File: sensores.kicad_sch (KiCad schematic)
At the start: 8 parts, among them U10 TCRT5000, U11 TCRT5000, U12 MPU-6050_module, U5 HC-Sr04, U6 HC-Sr04, U7 HC-Sr04, U8 KY-040, U9 KY-040

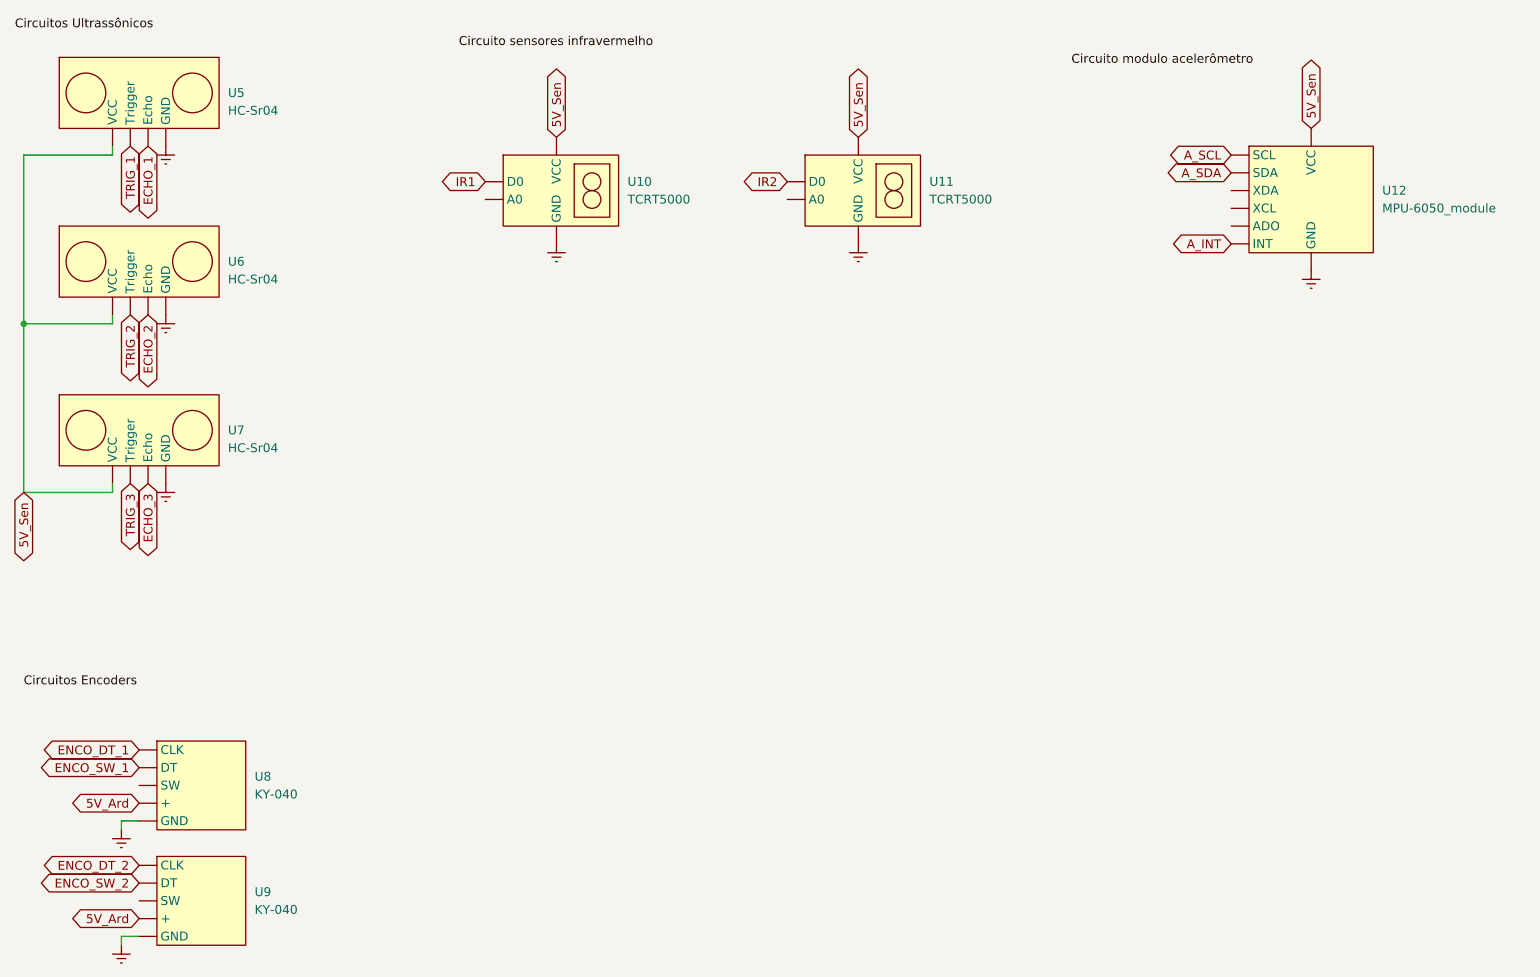
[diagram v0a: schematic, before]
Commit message: fix: esquematico atualizado
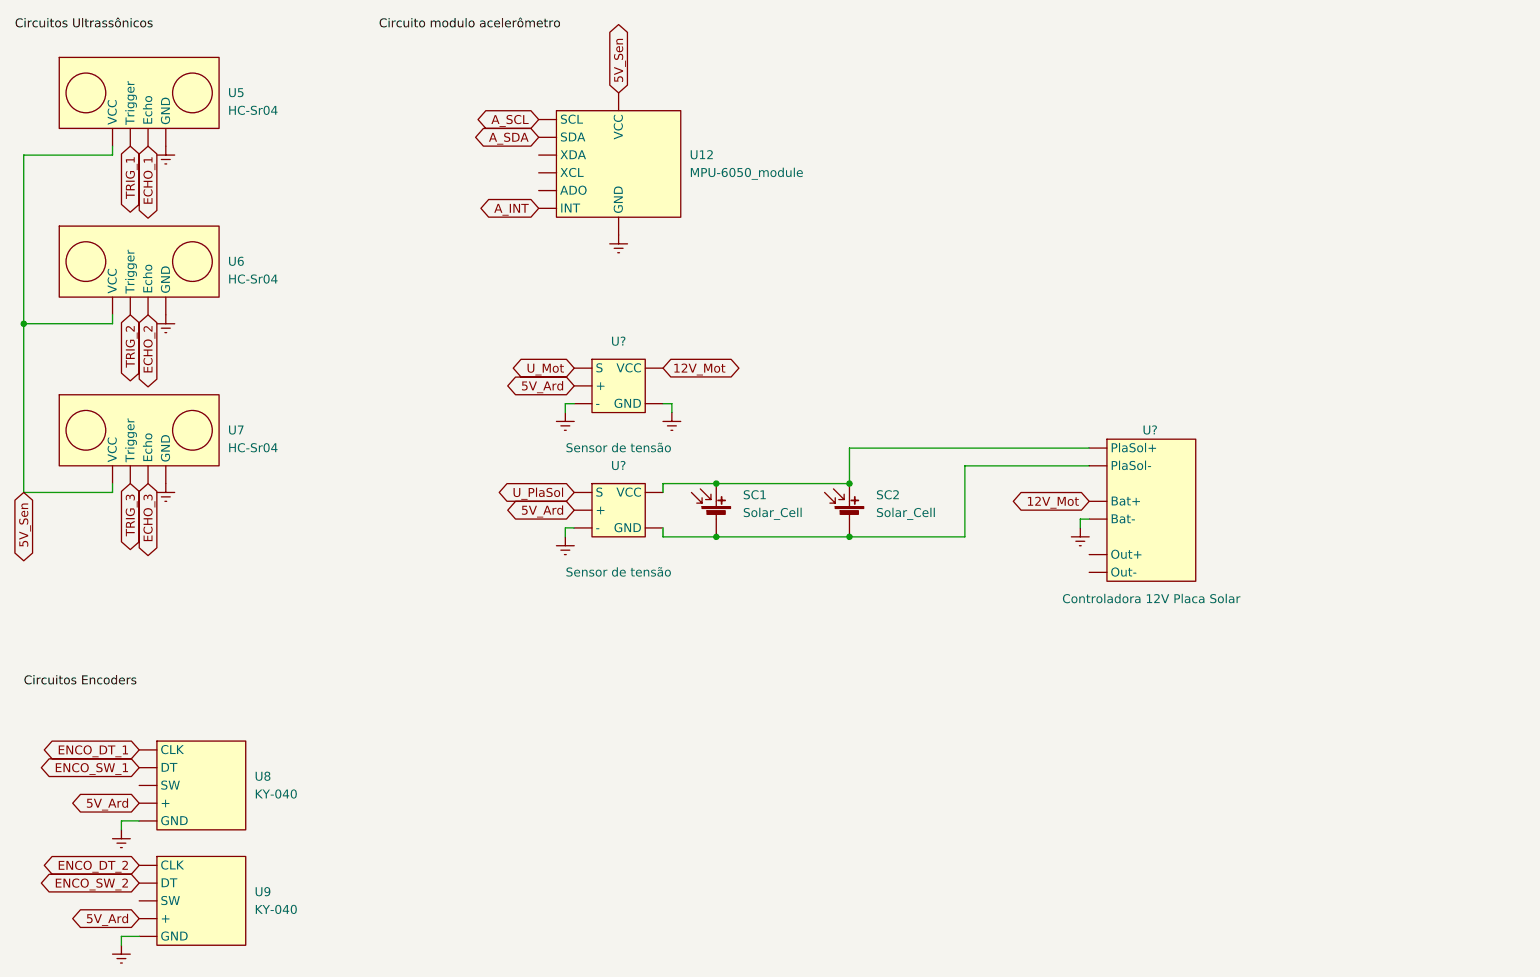
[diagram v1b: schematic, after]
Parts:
- removed U10, U11: TCRT5000, Connector_PinHeader_2.54mm:PinHeader_1x03_P2.54mm_Vertical, symbol Customizados:TCRT5000
- added SC1, SC2: Solar_Cell, symbol Device:Solar_Cell
- added U?: Controladora 12V Placa Solar, symbol Customizados:Controladora_12V_Placa_Solar
- added U? (x2): Sensor de tensão, symbol Customizados:Sensor_de_tensão
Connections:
- net 5V_Ard: now also U?. (VCC), U?. (VCC)
- net Earth: now also U?. (PlaSol-), U?. (VCC), U?. (VCC)
- new net: SC1.1 (+), SC2.1 (+), U?. (PlaSol-), U?. (VCC)
- new net: SC1.2 (-), SC2.2 (-), U?. (PlaSol-), U?. (VCC)
- new net 12V_Mot: U?. (PlaSol-), U?. (VCC)
- new net U_Mot: U?. (VCC)
- new net U_PlaSol: U?. (VCC)
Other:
- moved on the sheet: U12
